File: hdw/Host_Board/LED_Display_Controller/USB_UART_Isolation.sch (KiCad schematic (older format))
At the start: 8 parts

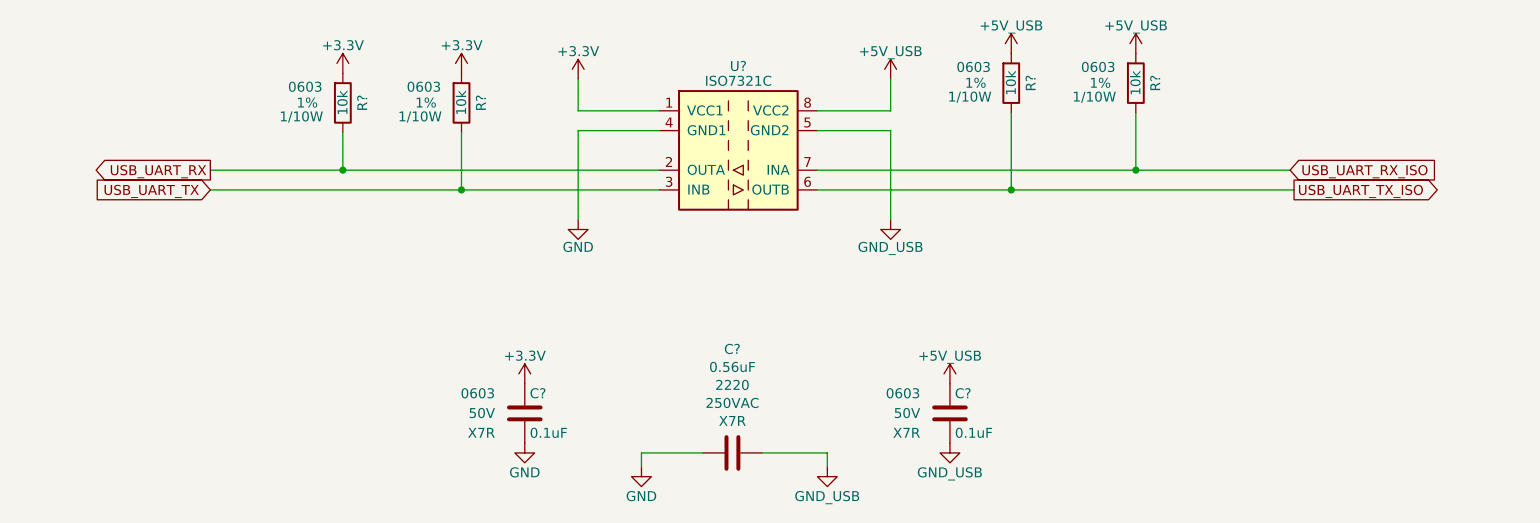
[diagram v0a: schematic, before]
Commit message: I said never do this, it's bad for you
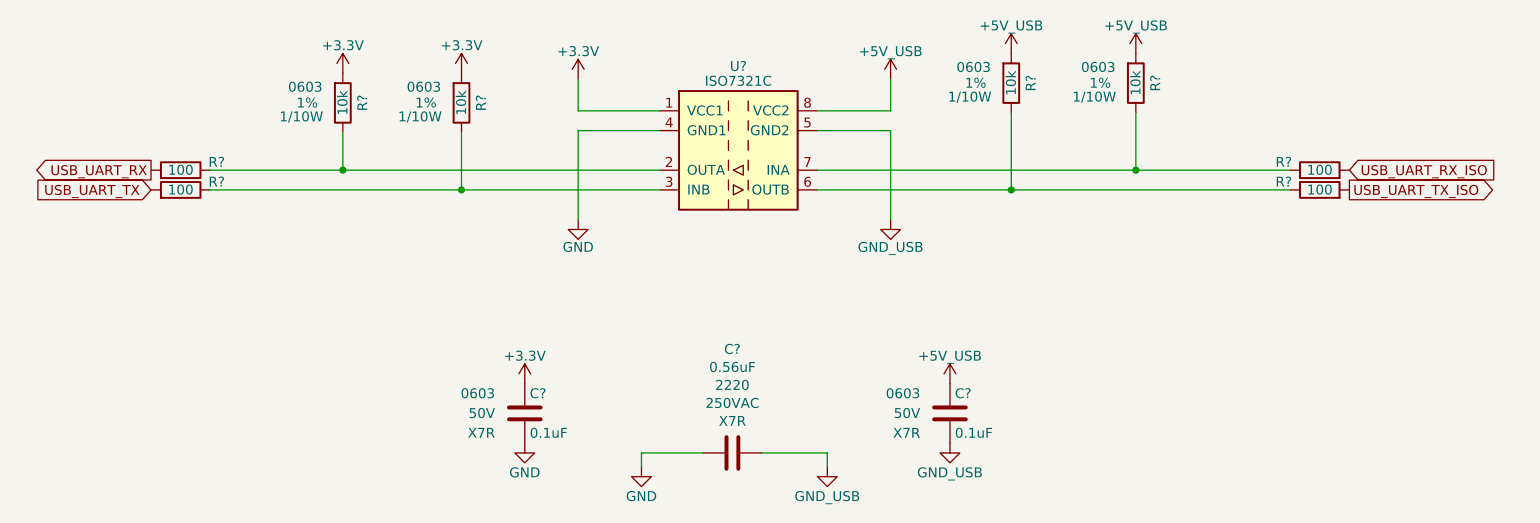
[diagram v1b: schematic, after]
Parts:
- added R? (x4): 100, symbol LED_Display_Local_Library:R_Custom
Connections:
- net USB_UART_RX: now also R?.1; no longer R?.2, U?.2 (OUTA)
- net USB_UART_RX_ISO: now also R?.1; no longer R?.2, U?.7 (INA)
- net USB_UART_TX: now also R?.1; no longer R?.2, U?.3 (INB)
- net USB_UART_TX_ISO: now also R?.1; no longer R?.2, U?.6 (OUTB)
- new net: R?.2, R?.2, U?.2 (OUTA)
- new net: R?.2, R?.2, U?.3 (INB)
- new net: R?.2, R?.2, U?.6 (OUTB)
- new net: R?.2, R?.2, U?.7 (INA)
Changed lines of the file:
@@
 $Descr A 11000 8500
 encoding utf-8
-Sheet 6 32
+Sheet 6 31
 Title ""
 Date ""
@@
 Comment4 ""
 $EndDescr
-Text GLabel 2850 3470 0    50   Output ~ 0
+Text GLabel 2550 3470 0    50   Output ~ 0
 USB_UART_RX
-Text GLabel 2850 3570 0    50   Input ~ 0
+Text GLabel 2550 3570 0    50   Input ~ 0
 USB_UART_TX
-Text GLabel 8310 3470 2    50   Input ~ 0
+Text GLabel 8610 3470 2    50   Input ~ 0
 USB_UART_RX_ISO
-Text GLabel 8330 3570 2    50   Output ~ 0
+Text GLabel 8610 3570 2    50   Output ~ 0
 USB_UART_TX_ISO
 $Comp
@@
 Connection ~ 6900 3570
 Wire Wire Line
-	6900 3570 8330 3570
+	6900 3570 8310 3570
 Wire Wire Line
 	7530 3180 7530 3470
@@
 Wire Wire Line
 	7530 3470 8310 3470
+$Comp
+L LED_Display_Local_Library:R_Custom R?
+U 1 1 5BE39290
+P 2700 3470
+AR Path="/5BAAE2B6/5BE39290" Ref="R?"  Part="1"
+AR Path="/5BB6CF6D/5BE39290" Ref="R?"  Part="1"
+AR Path="/5BBE424C/5BE39290" Ref="R?"  Part="1"
+AR Path="/5BAAE1DC/5BE39290" Ref="R?"  Part="1"
+F 0 "R?" V 2660 3330 50  0000 R CNN
+F 1 "100" V 2700 3470 50  0000 C CNN
+F 2 "" H 2700 3470 50  0001 C CNN
+F 3 "" H 2700 3470 50  0001 C CNN
+F 4 "0603" V 2800 3470 50  0001 C CNN "display_footprint"
+F 5 "1%" V 2900 3470 50  0001 C CNN "Tolerance"
+F 6 "1/10W" V 3000 3470 50  0001 C CNN "Wattage"
+F 7 "PN" H 3000 3870 60  0001 C CNN "Digi-Key PN"
+	1    2700 3470
+	0    -1   1    0
+$EndComp
+$Comp
+L LED_Display_Local_Library:R_Custom R?
+U 1 1 5BE3929B
+P 2700 3570
+AR Path="/5BAAE2B6/5BE3929B" Ref="R?"  Part="1"
+AR Path="/5BB6CF6D/5BE3929B" Ref="R?"  Part="1"
+AR Path="/5BBE424C/5BE3929B" Ref="R?"  Part="1"
+AR Path="/5BAAE1DC/5BE3929B" Ref="R?"  Part="1"
+F 0 "R?" V 2660 3430 50  0000 R CNN
+F 1 "100" V 2700 3570 50  0000 C CNN
+F 2 "" H 2700 3570 50  0001 C CNN
+F 3 "" H 2700 3570 50  0001 C CNN
+F 4 "0603" V 2800 3570 50  0001 C CNN "display_footprint"
+F 5 "1%" V 2900 3570 50  0001 C CNN "Tolerance"
+F 6 "1/10W" V 3000 3570 50  0001 C CNN "Wattage"
+F 7 "PN" H 3000 3970 60  0001 C CNN "Digi-Key PN"
+	1    2700 3570
+	0    -1   1    0
+$EndComp
+$Comp
+L LED_Display_Local_Library:R_Custom R?
+U 1 1 5BE39F31
+P 8460 3470
+AR Path="/5BAAE2B6/5BE39F31" Ref="R?"  Part="1"
+AR Path="/5BB6CF6D/5BE39F31" Ref="R?"  Part="1"
+AR Path="/5BBE424C/5BE39F31" Ref="R?"  Part="1"
+AR Path="/5BAAE1DC/5BE39F31" Ref="R?"  Part="1"
+F 0 "R?" V 8420 3330 50  0000 R CNN
+F 1 "100" V 8460 3470 50  0000 C CNN
+F 2 "" H 8460 3470 50  0001 C CNN
+F 3 "" H 8460 3470 50  0001 C CNN
+F 4 "0603" V 8560 3470 50  0001 C CNN "display_footprint"
+F 5 "1%" V 8660 3470 50  0001 C CNN "Tolerance"
+F 6 "1/10W" V 8760 3470 50  0001 C CNN "Wattage"
+F 7 "PN" H 8760 3870 60  0001 C CNN "Digi-Key PN"
+	1    8460 3470
+	0    1    1    0
+$EndComp
+$Comp
+L LED_Display_Local_Library:R_Custom R?
+U 1 1 5BE39F3C
+P 8460 3570
+AR Path="/5BAAE2B6/5BE39F3C" Ref="R?"  Part="1"
+AR Path="/5BB6CF6D/5BE39F3C" Ref="R?"  Part="1"
+AR Path="/5BBE424C/5BE39F3C" Ref="R?"  Part="1"
+AR Path="/5BAAE1DC/5BE39F3C" Ref="R?"  Part="1"
+F 0 "R?" V 8420 3430 50  0000 R CNN
+F 1 "100" V 8460 3570 50  0000 C CNN
+F 2 "" H 8460 3570 50  0001 C CNN
+F 3 "" H 8460 3570 50  0001 C CNN
+F 4 "0603" V 8560 3570 50  0001 C CNN "display_footprint"
+F 5 "1%" V 8660 3570 50  0001 C CNN "Tolerance"
+F 6 "1/10W" V 8760 3570 50  0001 C CNN "Wattage"
+F 7 "PN" H 8760 3970 60  0001 C CNN "Digi-Key PN"
+	1    8460 3570
+	0    1    1    0
+$EndComp
 $EndSCHEMATC
